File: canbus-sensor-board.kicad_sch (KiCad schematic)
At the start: 48 parts, among them J1 CAN IO, J2 CAN Term, J3 POWER IN, J4 Debug, J5 I2C2 IO, J6 I2C1 IO, Q1 2N7002, Q2 2N7002, Q3 2N7002, Q4 2N7002, SW1 Reset, SW2 Boot, U1 MCP2551-I-SN, U3 AMS1117-3.3, U4 STM32F103C8Tx

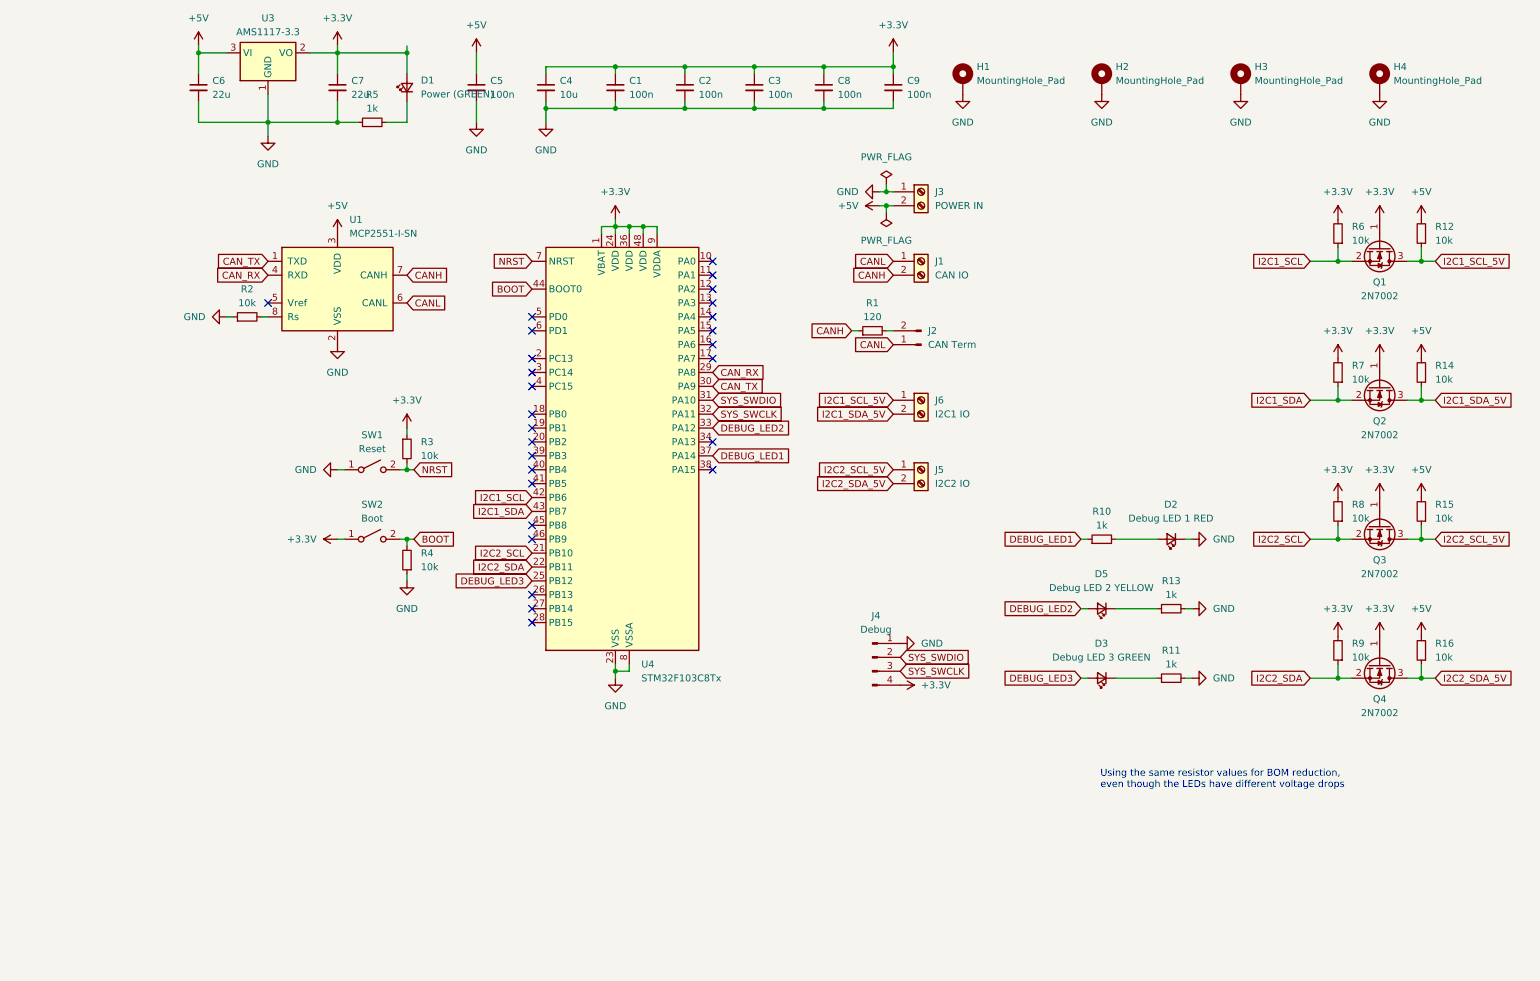
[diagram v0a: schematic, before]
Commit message: Update board to rev 3 (we do not talk about rev 2)
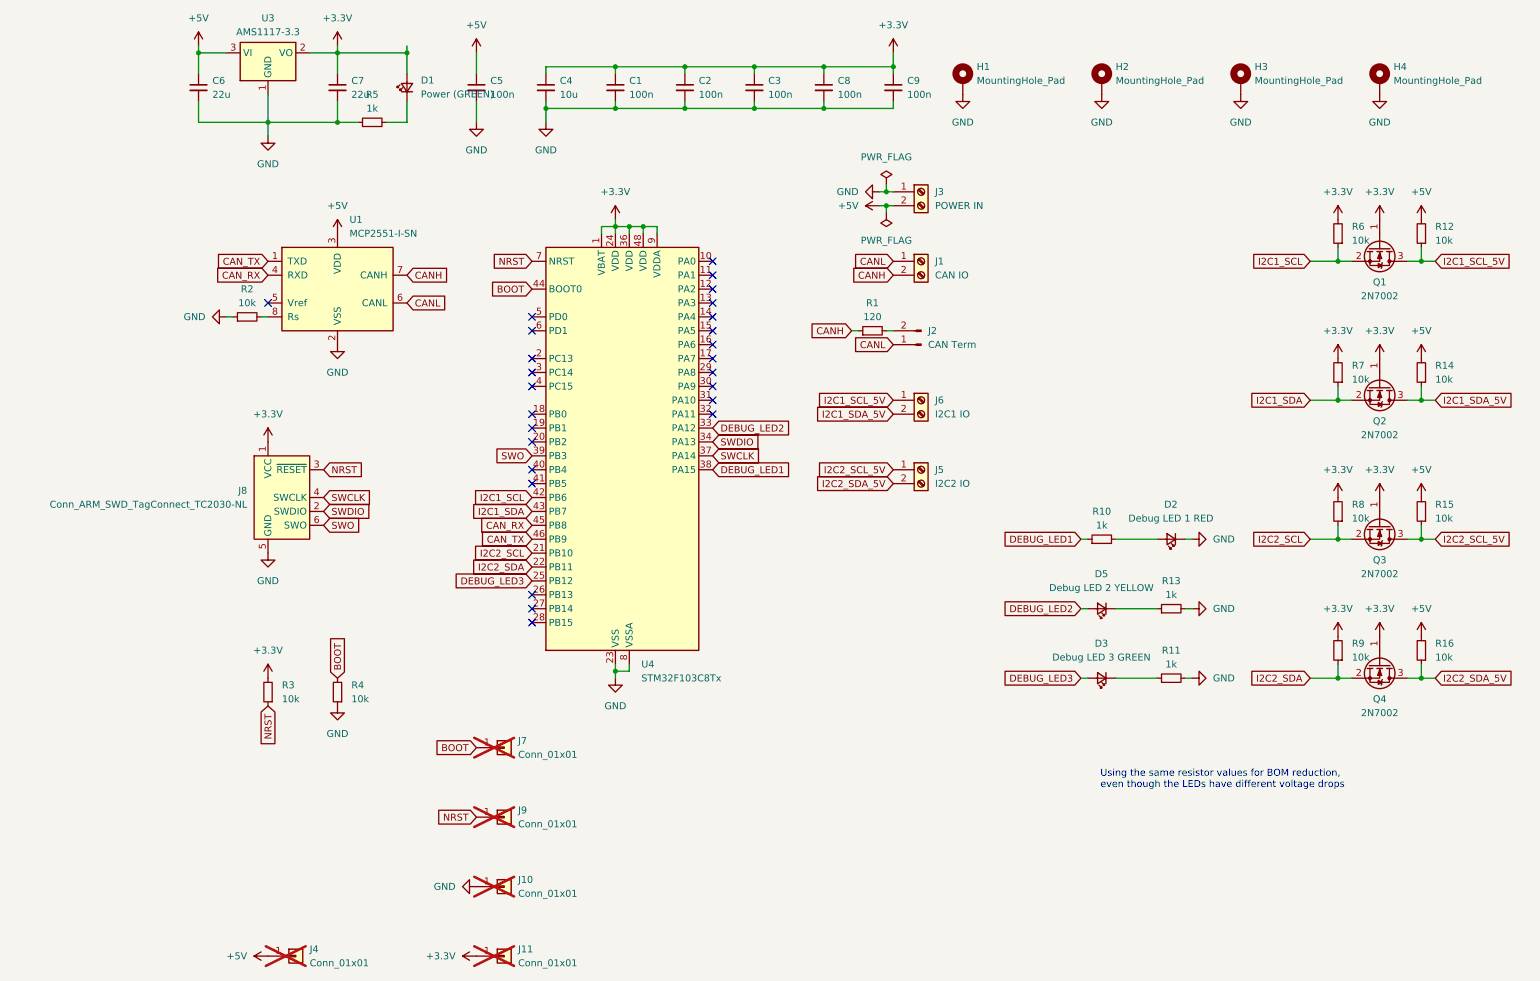
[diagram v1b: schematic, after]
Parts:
- removed J4: Debug, Connector_PinHeader_2.54mm:PinHeader_1x04_P2.54mm_Vertical, symbol Connector:Conn_01x04_Pin
- removed SW1: Reset, Button_Switch_SMD:SW_Push_1P1T_XKB_TS-1187A, symbol Switch:SW_SPST
- removed SW2: Boot, Button_Switch_SMD:SW_Push_1P1T_XKB_TS-1187A, symbol Switch:SW_SPST
- added J10, J11, J4, J7, J9: Conn_01x01, Connector_Wire:SolderWirePad_1x01_SMD_1x2mm, symbol Connector_Generic:Conn_01x01
- added J8: Conn_ARM_SWD_TagConnect_TC2030-NL, Connector:Tag-Connect_TC2030-IDC-NL_2x03_P1.27mm_Vertical, symbol Connector:Conn_ARM_SWD_TagConnect_TC2030-NL
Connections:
- net +3.3V: now also R3.2, J11.1 (Pin_1), J8.1 (VCC); no longer R3.1
- net +5V: now also J4.1 (Pin_1)
- net BOOT: now also J7.1 (Pin_1)
- net CAN_RX: now also U4.45 (PB8); no longer U4.29 (PA8)
- net CAN_TX: now also U4.46 (PB9); no longer U4.30 (PA9)
- net DEBUG_LED1: now also U4.38 (PA15); no longer U4.37 (PA14)
- net GND: now also J10.1 (Pin_1), J8.5 (GND)
- net NRST: now also R3.1, J8.3 (~{RESET}), J9.1 (Pin_1); no longer R3.2
- net SWDIO: now reaches U4.34 (PA13)
- net SWDIO: now also J8.2 (SWDIO)
- net SWO: now reaches U4.39 (PB3)
- net SWO: now also J8.6 (SWO)
- net SYS_SWCLK: no longer names the net of U4.32 (PA11)
- net SYS_SWDIO: no longer names the net of U4.31 (PA10)
- new net SWCLK: J8.4 (SWCLK), U4.37 (PA14)
- no-connect marks 27 -> 26
